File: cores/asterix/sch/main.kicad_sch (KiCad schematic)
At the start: 25 parts

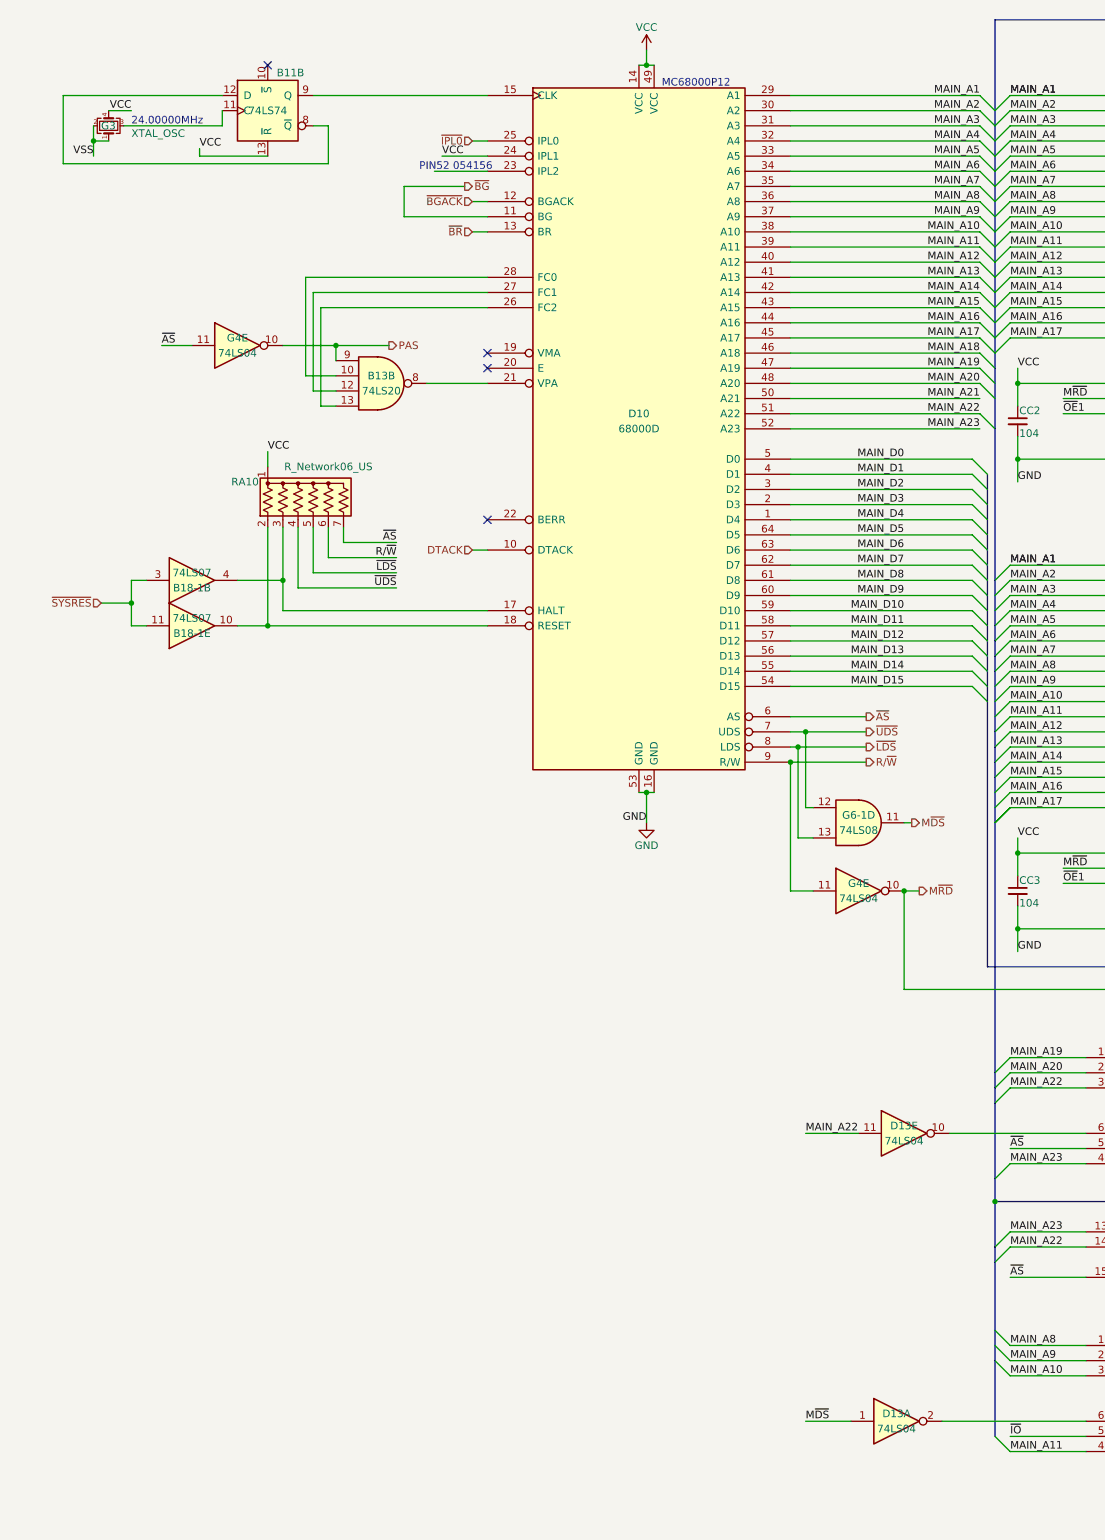
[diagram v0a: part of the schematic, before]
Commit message: wip scr. wip custom chips konami 054156 57
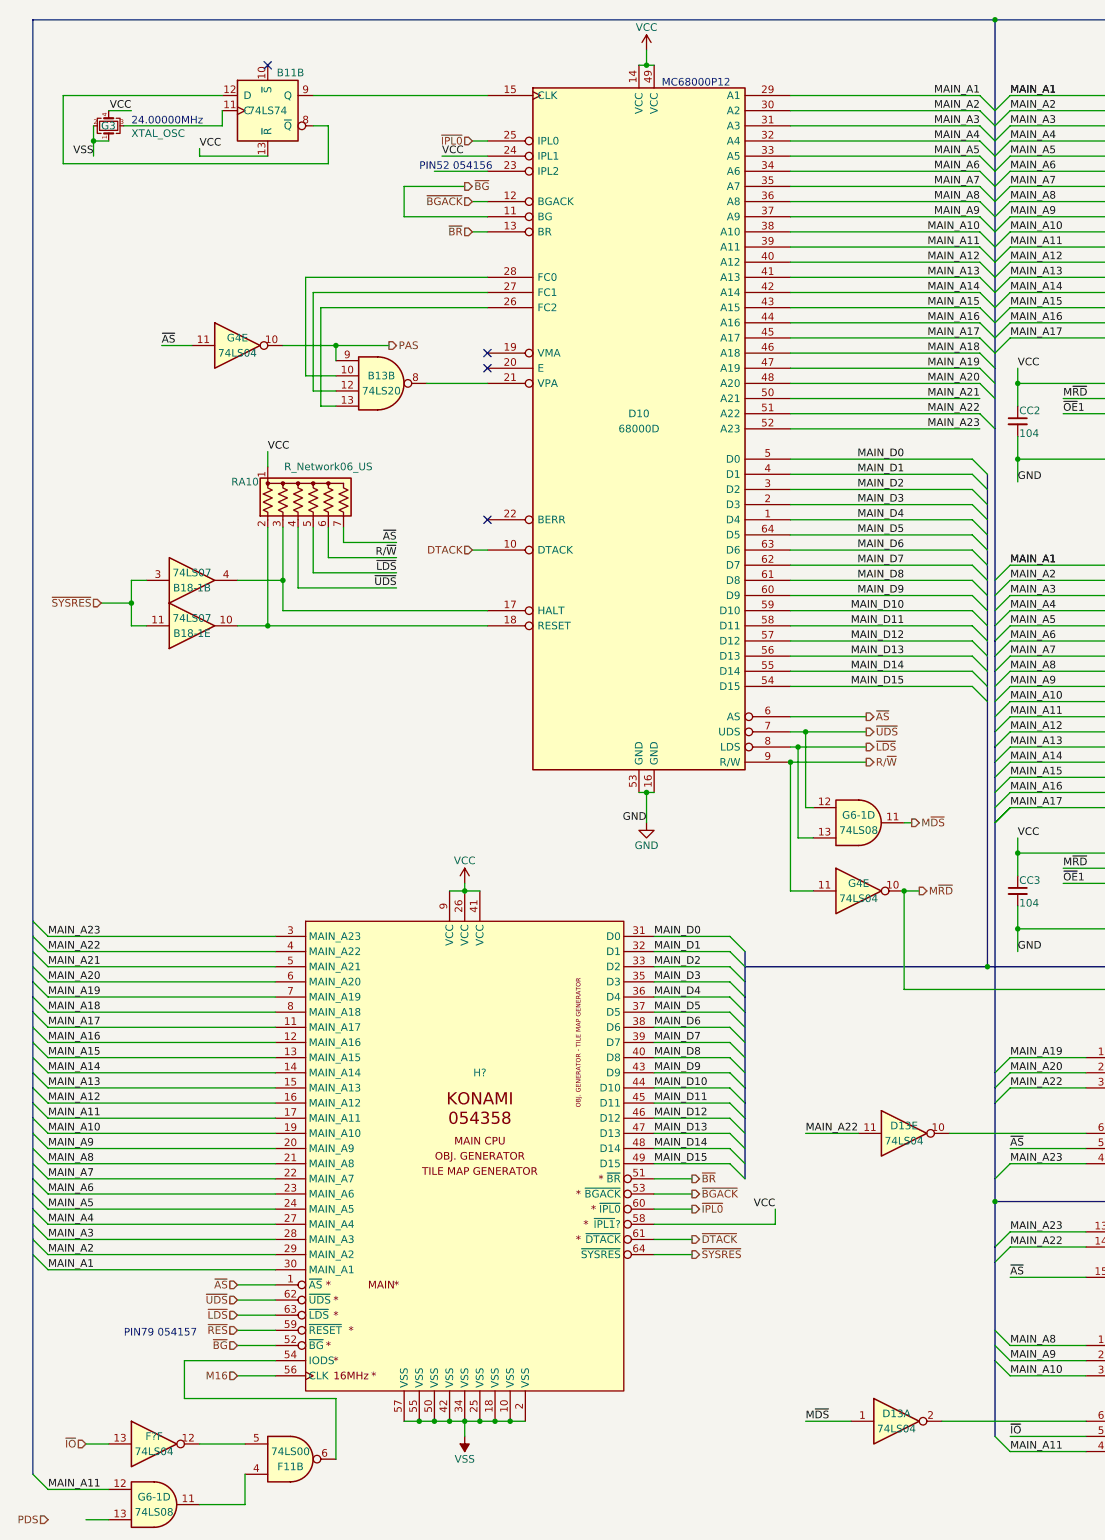
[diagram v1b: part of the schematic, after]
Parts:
- added F11: 74LS00, symbol jt74:74LS00
- added F?: 74LS04, symbol jt74:74LS04
- added G6-1: 74LS08, symbol jt74:74LS08
- added H?: ~, symbol konami:054358
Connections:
- net MAIN_A1: now also H?.30 (MAIN_A1)
- net MAIN_A10: now also H?.19 (MAIN_A10)
- net MAIN_A11: now also G6-1.12, H?.17 (MAIN_A11)
- net MAIN_A12: now also H?.16 (MAIN_A12)
- net MAIN_A13: now also H?.15 (MAIN_A13)
- net MAIN_A14: now also H?.14 (MAIN_A14)
- net MAIN_A15: now also H?.13 (MAIN_A15)
- net MAIN_A16: now also H?.12 (MAIN_A16)
- net MAIN_A17: now also H?.11 (MAIN_A17)
- net MAIN_A18: now also H?.8 (MAIN_A18)
- net MAIN_A19: now also H?.7 (MAIN_A19)
- net MAIN_A2: now also H?.29 (MAIN_A2)
- net MAIN_A20: now also H?.6 (MAIN_A20)
- net MAIN_A21: now also H?.5 (MAIN_A21)
- net MAIN_A22: now also H?.4 (MAIN_A22)
- net MAIN_A23: now also H?.3 (MAIN_A23)
- net MAIN_A3: now also H?.28 (MAIN_A3)
- net MAIN_A4: now also H?.27 (MAIN_A4)
- net MAIN_A5: now also H?.24 (MAIN_A5)
- net MAIN_A6: now also H?.23 (MAIN_A6)
- net MAIN_A7: now also H?.22 (MAIN_A7)
- net MAIN_A8: now also H?.21 (MAIN_A8)
- net MAIN_A9: now also H?.20 (MAIN_A9)
- net MAIN_D0: now also H?.31 (D0)
- net MAIN_D1: now also H?.32 (D1)
- net MAIN_D10: now also H?.44 (D10)
- net MAIN_D11: now also H?.45 (D11)
- net MAIN_D12: now also H?.46 (D12)
- net MAIN_D13: now also H?.47 (D13)
- net MAIN_D14: now also H?.48 (D14)
- net MAIN_D15: now also H?.49 (D15)
- net MAIN_D2: now also H?.33 (D2)
- net MAIN_D3: now also H?.35 (D3)
- net MAIN_D4: now also H?.36 (D4)
- net MAIN_D5: now also H?.37 (D5)
- net MAIN_D6: now also H?.38 (D6)
- net MAIN_D7: now also H?.39 (D7)
- net MAIN_D8: now also H?.40 (D8)
- net MAIN_D9: now also H?.43 (D9)
- net VCC: now also H?.26 (VCC), H?.41 (VCC), H?.58 (~{IPL1}?), H?.9 (VCC)
- net VSS: now also H?.10 (VSS), H?.18 (VSS), H?.2 (VSS), H?.25 (VSS), H?.34 (VSS), H?.42 (VSS), H?.50 (VSS), H?.55 (VSS), H?.57 (VSS)
- net ~{AS}: now also H?.1 (~{AS})
- net ~{BGACK}: now also H?.53 (~{BGACK})
- net ~{BG}: now also H?.52 (~{BG})
- net ~{BR}: now also H?.51 (~{BR})
- net ~{IO}: now also F?.13
- net ~{IPL0}: now also H?.60 (~{IPL0})
- net ~{LDS}: now also H?.63 (~{LDS})
- net ~{SYSRES}: now also H?.64 (~{SYSRES})
- net ~{UDS}: now also H?.62 (~{UDS})
- new net: F11.4, G6-1.11
- new net: F11.5, F?.12
- new net: F11.6, H?.54 (IODS)
- new net M16: H?.56 (CLK)
- new net ~{DTACK}: H?.61 (~{DTACK})
- new net ~{RES}: H?.59 (~{RESET})
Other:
- note added: "PIN79 054157"
